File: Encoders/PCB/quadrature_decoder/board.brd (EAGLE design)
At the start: 84.8 x 55.9 mm, 14 parts, among them IC1 LFLS7366R, IC2 LFLS7366R, IC3 LFLS7366R, IC4 LFLS7366R, IC5 LFLS7366R, IC6 LFLS7366R

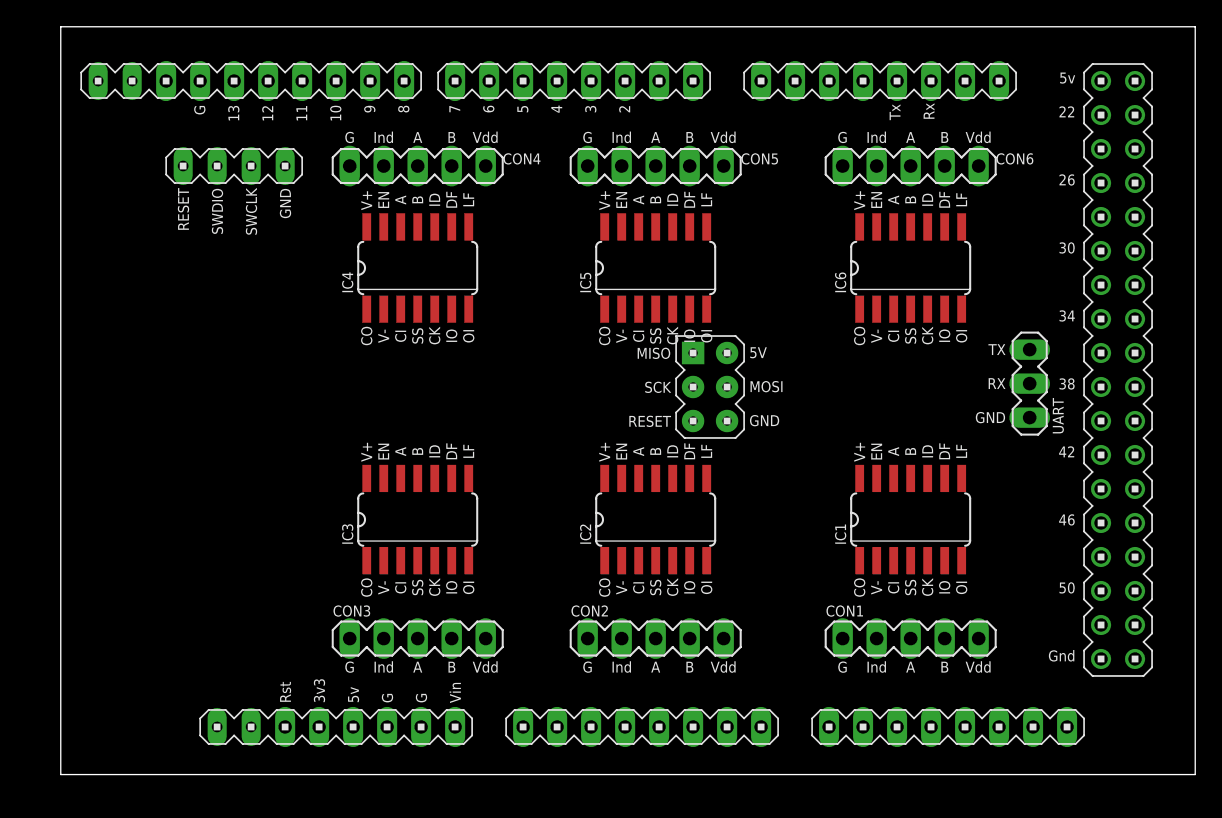
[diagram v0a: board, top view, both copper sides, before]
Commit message: new board
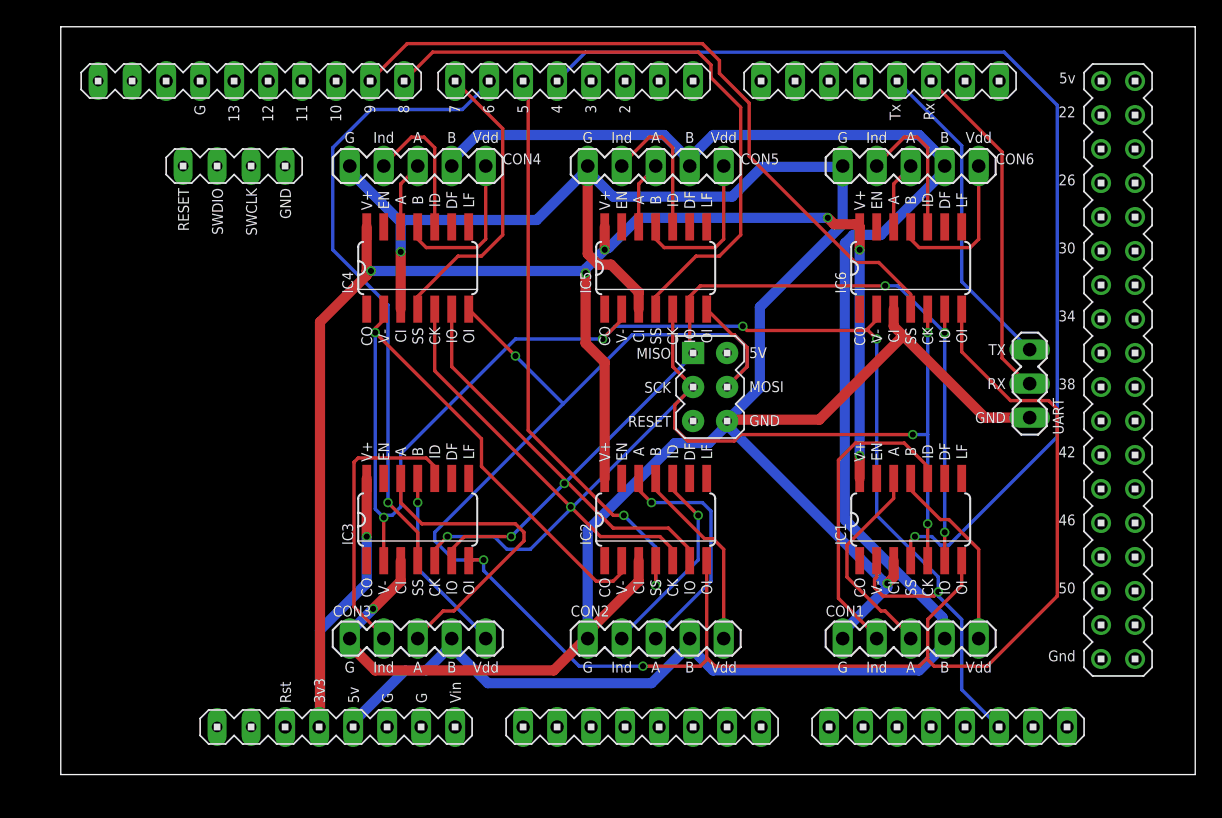
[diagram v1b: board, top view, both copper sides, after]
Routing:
- net GND: track 0.00 -> 196.1 mm, vias 0 -> 3
- net MOSI: track 0.00 -> 148.8 mm, vias 0 -> 3
- net FCKI: track 0.00 -> 138.1 mm, vias 0 -> 6
- net 5V: track 0.00 -> 137.7 mm
- net 3.3V: track 0.00 -> 134.3 mm, vias 0 -> 7
- net SCK: track 0.00 -> 103.2 mm, vias 0 -> 5
- net MISO: track 0.00 -> 97.9 mm, vias 0 -> 5
- net SS1: track 0.00 -> 80.9 mm, vias 0 -> 1
- net SS6: track 0.00 -> 53.3 mm
- net SS3: track 0.00 -> 47.4 mm, vias 0 -> 1
- net SS5: track 0.00 -> 47.0 mm
- net SS2: track 0.00 -> 44.1 mm, vias 0 -> 2
- net N$4: track 0.00 -> 25.8 mm
- net N$3: track 0.00 -> 24.2 mm
- net N$9: track 0.00 -> 23.6 mm
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
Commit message: rerouted
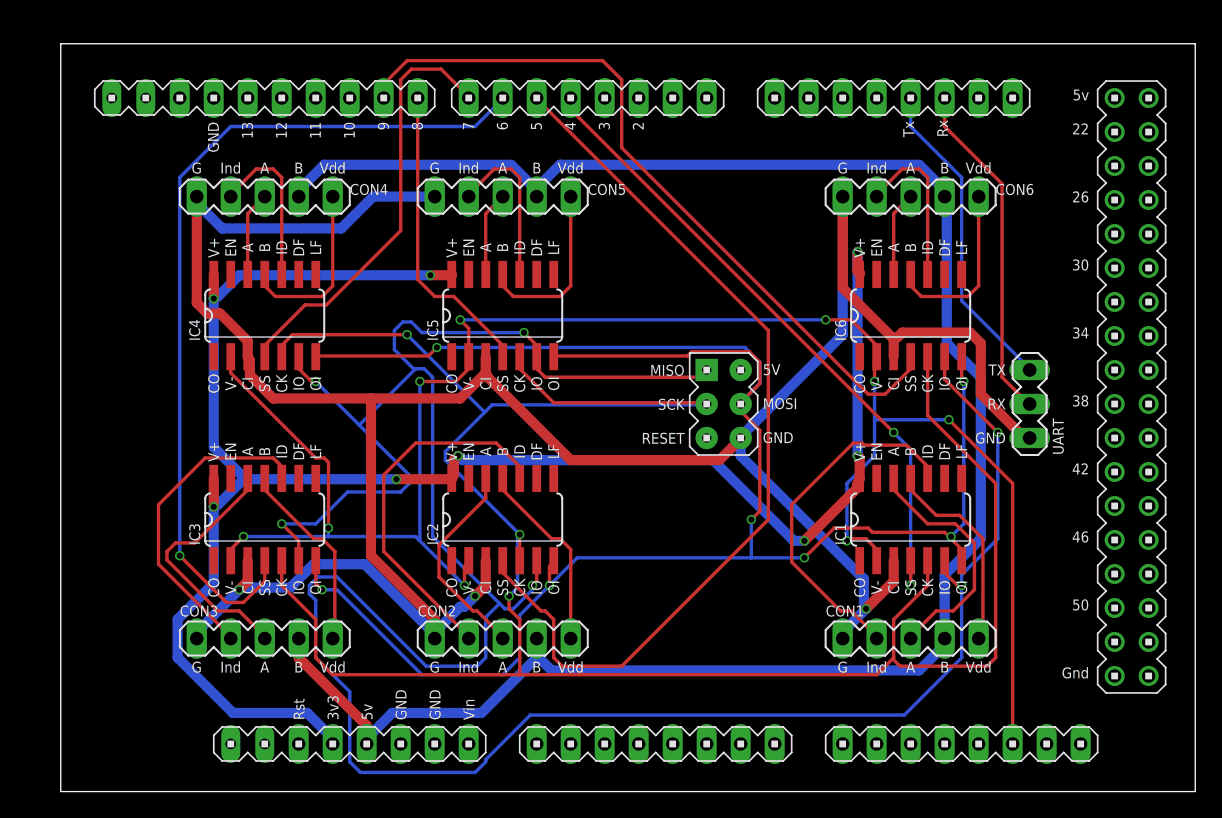
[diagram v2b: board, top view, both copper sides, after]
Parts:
- moved IC4 12.0 mm to (17.8, 35.6)
- moved IC5 12.0 mm to (35.6, 35.6)
- moved CON4 11.7 mm to (17.8, 44.5)
- moved CON5 11.7 mm to (35.6, 44.5)
- moved CON2 11.4 mm to (35.6, 11.4)
- moved CON3 11.4 mm to (17.8, 11.4)
- moved IC2 11.4 mm to (35.6, 20.3)
- moved IC3 11.4 mm to (17.8, 20.3)
- moved IC6 3.56 mm to (66.0, 35.6)
- moved CON6 2.29 mm to (66.0, 44.5)
- moved U$1 1.63 mm to (62.2, 21.3)
- moved UART 1.52 mm to (74.9, 29.0)
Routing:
- net MISO: track 97.9 -> 202.1 mm, vias 5 -> 6
- net SCK: track 103.2 -> 171.1 mm, vias 5 -> 3
- net SS1: track 80.9 -> 48.8 mm, vias 1 -> 2
- net SS2: track 44.1 -> 68.5 mm, vias 2 -> 0
- net SS5: track 47.0 -> 22.8 mm
- net SS3: track 47.4 -> 64.9 mm
- net N$2: track 15.1 -> 27.6 mm, vias 1 -> 0
- net 5V: track 137.7 -> 147.7 mm
- net SS4: track 22.2 -> 32.2 mm
- net GND: track 196.1 -> 205.7 mm
- net N$9: track 23.6 -> 19.3 mm
- net 3.3V: track 134.3 -> 137.9 mm, vias 7 -> 8
- net N$12: track 23.3 -> 26.8 mm
- net FCKI: track 138.1 -> 141.5 mm, vias 6 -> 9
- net SS6: track 53.3 -> 56.1 mm
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
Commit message: updated board
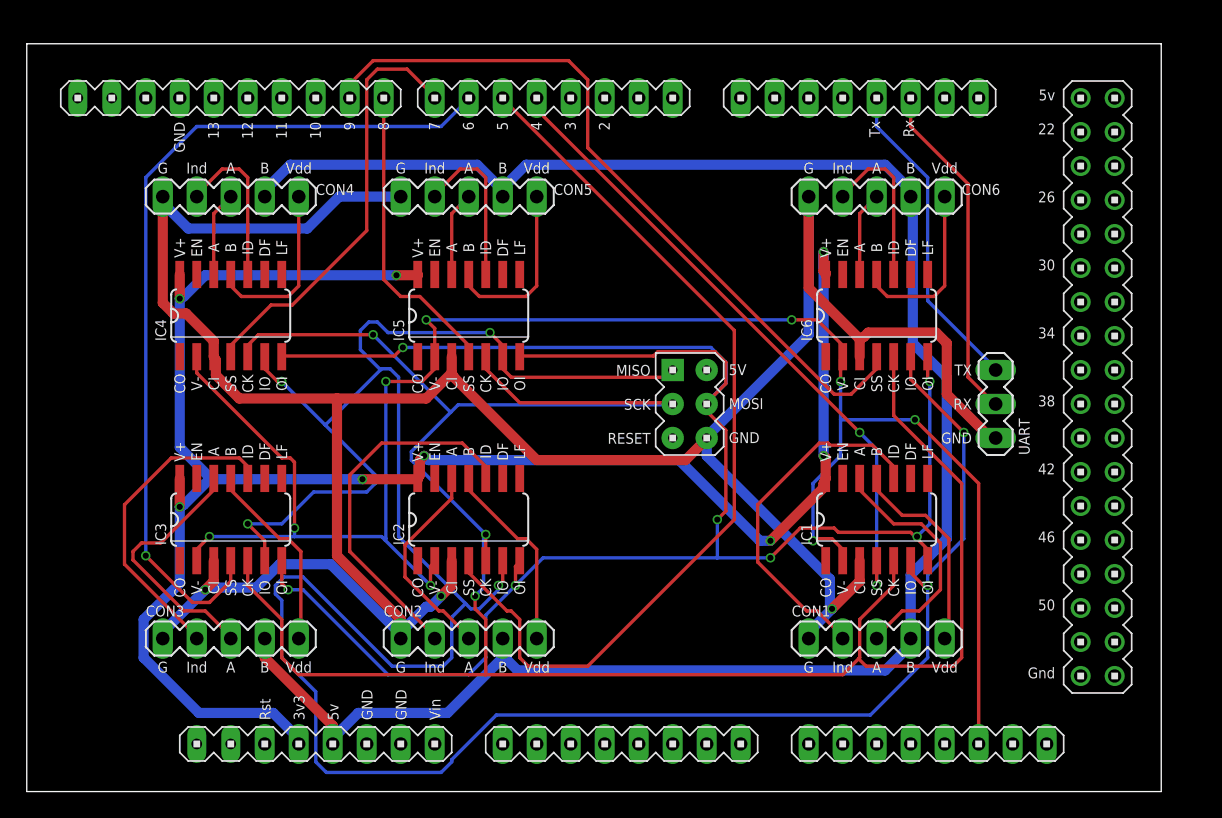
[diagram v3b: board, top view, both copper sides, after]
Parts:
- moved CON1 2.54 mm to (63.5, 11.4)
- moved CON6 2.54 mm to (63.5, 44.5)
- moved IC1 2.54 mm to (63.5, 20.3)
- moved IC6 2.54 mm to (63.5, 35.6)
- moved UART 2.54 mm to (72.4, 29.0)
- moved CON3 2.54 mm to (15.2, 11.4)
- moved CON4 2.54 mm to (15.2, 44.5)
- moved IC3 2.54 mm to (15.2, 20.3)
- moved IC4 2.54 mm to (15.2, 35.6)
- moved CON2 2.54 mm to (33.0, 11.4)
- moved CON5 2.54 mm to (33.0, 44.5)
- moved IC2 2.54 mm to (33.0, 20.3)
- moved IC5 2.54 mm to (33.0, 35.6)
- moved U$1 2.54 mm to (59.7, 21.3)
